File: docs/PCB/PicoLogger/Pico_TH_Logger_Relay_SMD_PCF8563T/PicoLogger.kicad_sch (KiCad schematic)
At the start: 63 parts, among them J1 Sensor, J2 LCD 16x2, J3 Additional connector, J4 K4_Output, J5 K3_Output, J6 K2_Output, J7 K1_Output, J8 SPI, K1 G5Q-1, K2 G5Q-1, K3 G5Q-1, K4 G5Q-1, Q1 MMBT3904, Q2 MMBT3904, Q3 MMBT3904, Q4 MMBT3904, SW1 SW_Push, SW2 SW_Push, U1 LTV-817S, U2 LTV-817S, U3 LTV-817S, U4 LTV-817S, U5 PCF8563T, Y1 Crystal

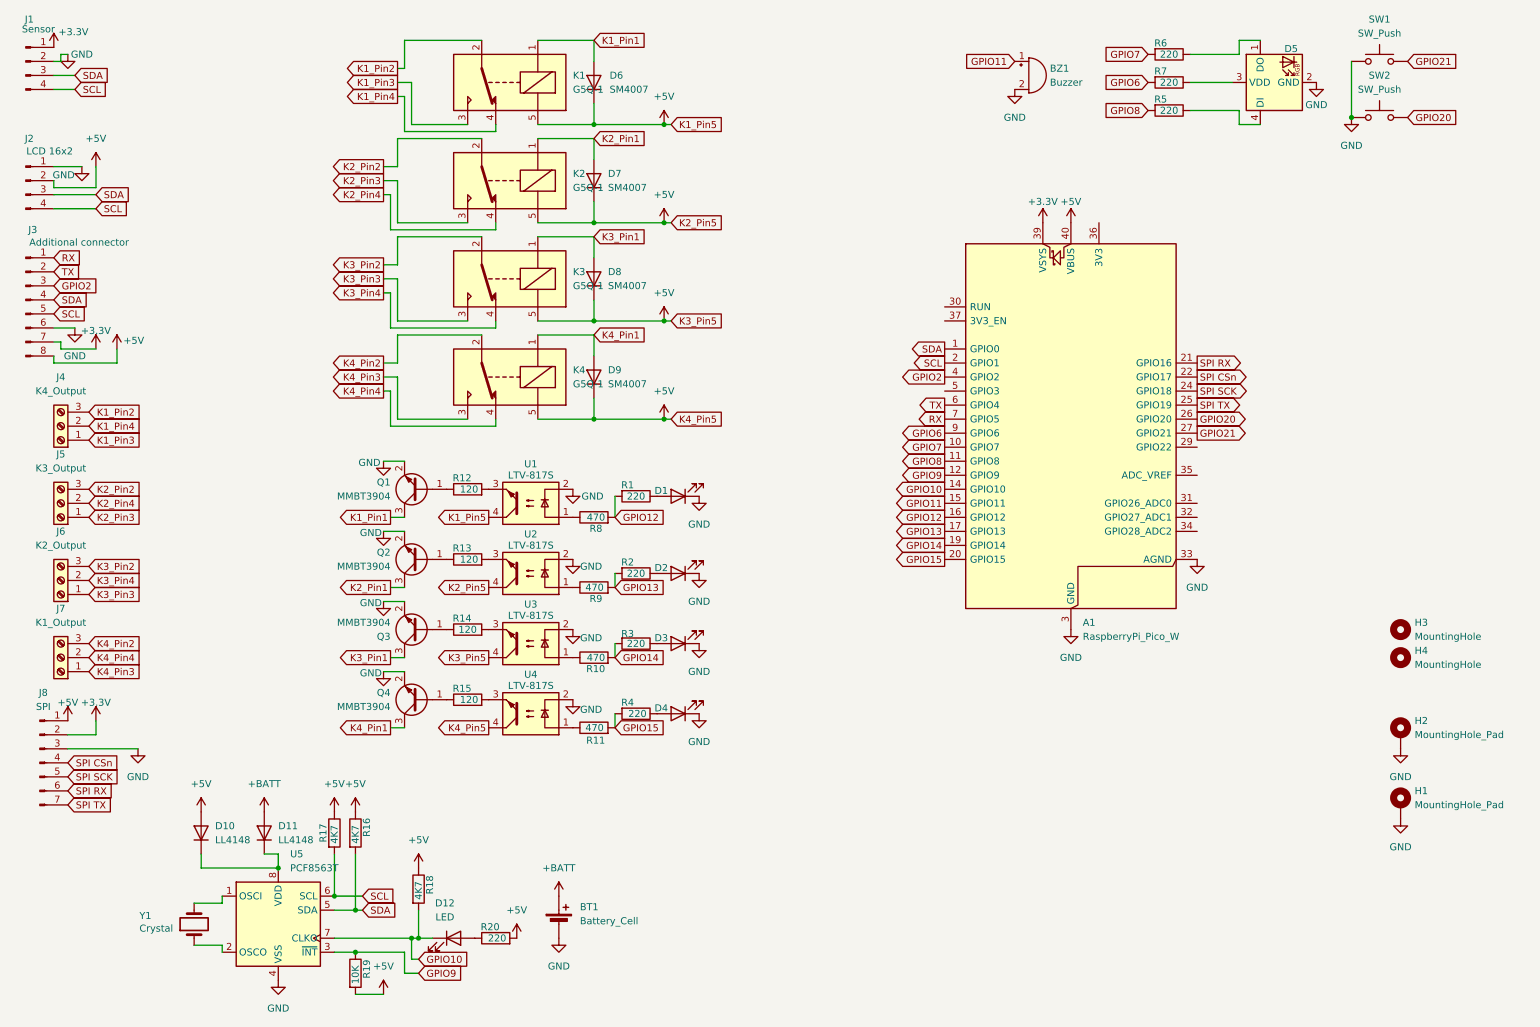
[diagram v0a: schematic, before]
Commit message: Updated docs.
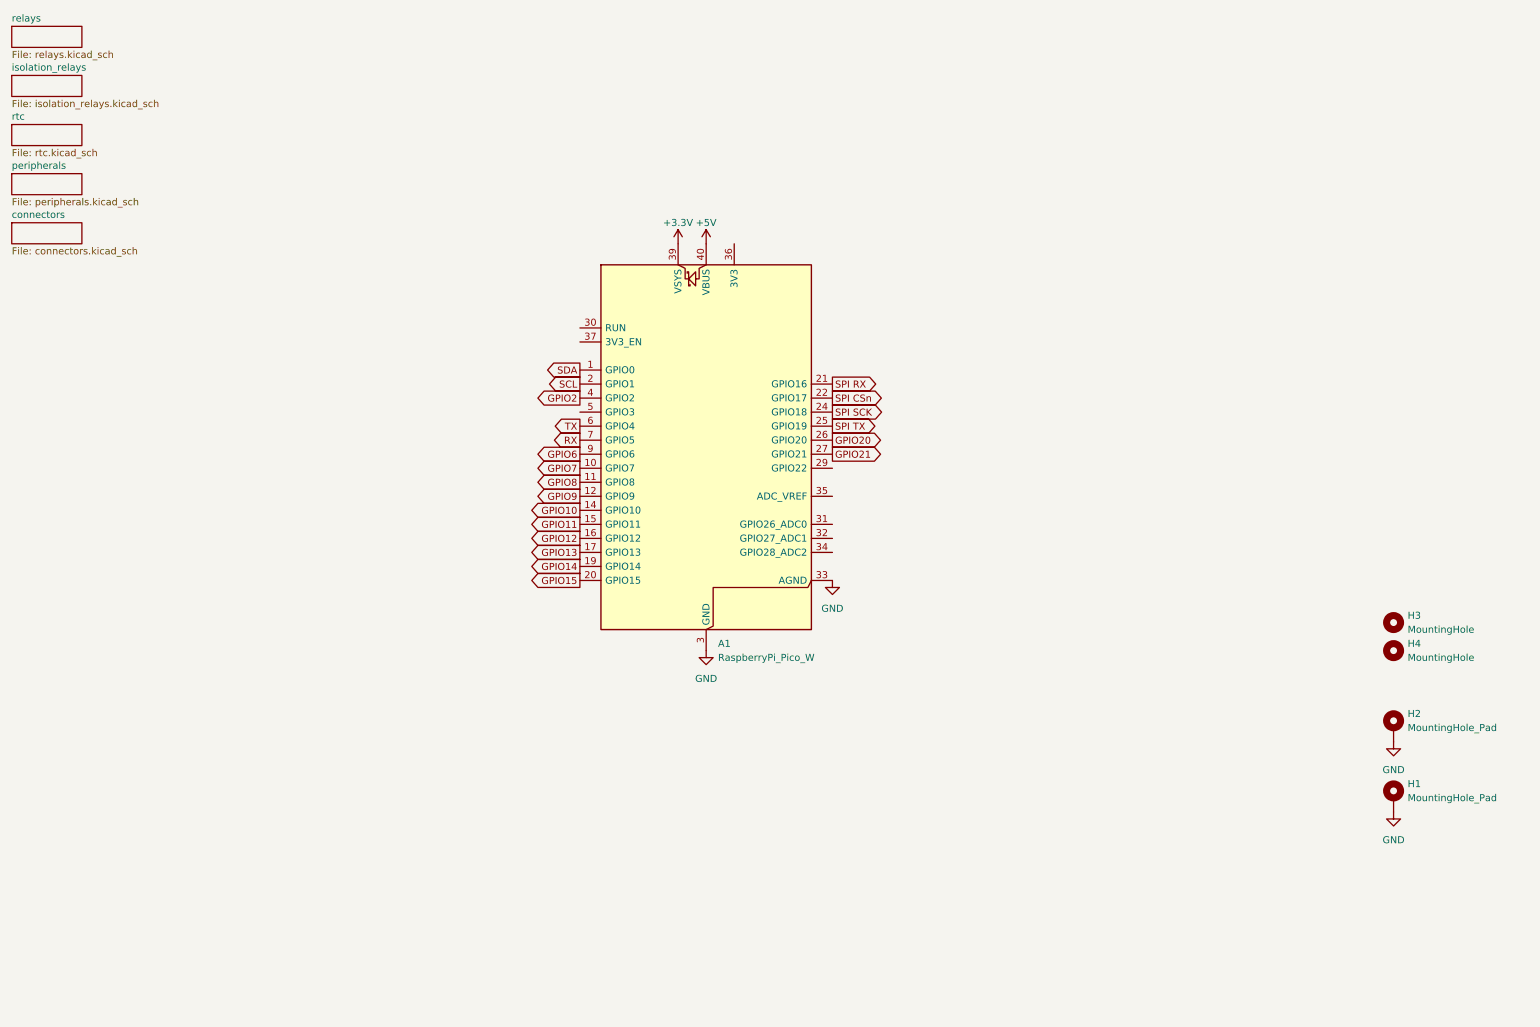
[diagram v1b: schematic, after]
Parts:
- removed BT1: Battery_Cell, Battery:BatteryHolder_Keystone_104_1x23mm, symbol Device:Battery_Cell
- removed BZ1: Buzzer, Buzzer_Beeper:Buzzer_12x9.5RM7.6, symbol Device:Buzzer
- removed D1, D12, D2, D3, D4: LED, LED_SMD:LED_0805_2012Metric, symbol Device:LED
- removed D10, D11: LL4148, Diode_SMD:D_MiniMELF, symbol Diode:LL4148
- removed D5: APA-106-F5, LED_SMD:LED_Avago_PLCC4_3.2x2.8mm_CW, symbol LED:APA-106-F5
- removed D6, D7, D8, D9: SM4007, Diode_SMD:D_SMA, symbol Diode:SM4007
- removed J1: Sensor, Connector_PinHeader_2.54mm:PinHeader_1x04_P2.54mm_Vertical, symbol Connector:Conn_01x04_Pin
- removed J2: LCD 16x2, Connector_PinHeader_2.54mm:PinHeader_1x04_P2.54mm_Vertical, symbol Connector:Conn_01x04_Pin
- removed J3: Additional connector, Connector_PinHeader_2.54mm:PinHeader_1x08_P2.54mm_Horizontal, symbol Connector:Conn_01x08_Pin
- removed J4: K4_Output, TerminalBlock_Phoenix:TerminalBlock_Phoenix_MKDS-1,5-3_1x03_P5.00mm_Horizontal, symbol Connector:Screw_Terminal_01x03
- removed J5: K3_Output, TerminalBlock_Phoenix:TerminalBlock_Phoenix_MKDS-1,5-3_1x03_P5.00mm_Horizontal, symbol Connector:Screw_Terminal_01x03
- removed J6: K2_Output, TerminalBlock_Phoenix:TerminalBlock_Phoenix_MKDS-1,5-3_1x03_P5.00mm_Horizontal, symbol Connector:Screw_Terminal_01x03
- removed J7: K1_Output, TerminalBlock_Phoenix:TerminalBlock_Phoenix_MKDS-1,5-3_1x03_P5.00mm_Horizontal, symbol Connector:Screw_Terminal_01x03
- removed J8: SPI, Connector_PinHeader_2.54mm:PinHeader_1x07_P2.54mm_Horizontal, symbol Connector:Conn_01x07_Pin
- removed K1, K2, K3, K4: G5Q-1, Relay_THT:Relay_SPDT_Omron-G5Q-1, symbol Relay:G5Q-1
- removed Q1, Q2, Q3, Q4: MMBT3904, Package_TO_SOT_SMD:SOT-23, symbol Transistor_BJT:MMBT3904
- removed R1, R2, R20, R3, R4, R5, R6, R7: 220, Resistor_SMD:R_0805_2012Metric, symbol Device:R
- removed R10, R11, R8, R9: 470, Resistor_SMD:R_0805_2012Metric, symbol Device:R
- removed R12, R13, R14, R15: 120, Resistor_SMD:R_0805_2012Metric, symbol Device:R
- removed R16, R17, R18: 4K7, Resistor_SMD:R_0805_2012Metric, symbol Device:R
- removed R19: 10K, Resistor_SMD:R_0805_2012Metric, symbol Device:R
- removed SW1, SW2: SW_Push, Button_Switch_THT:SW_PUSH_6mm, symbol Switch:SW_Push
- removed U1, U2, U3, U4: LTV-817S, Package_DIP:SMDIP-4_W9.53mm, symbol Isolator:LTV-817S
- removed U5: PCF8563T, Package_SO:SOIC-8_3.9x4.9mm_P1.27mm, symbol Timer_RTC:PCF8563T
- removed Y1: Crystal, Crystal:Crystal_SMD_3215-2Pin_3.2x1.5mm, symbol Device:Crystal
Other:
- added sheet connectors (connectors.kicad_sch)
- added sheet isolation_relays (isolation_relays.kicad_sch)
- added sheet peripherals (peripherals.kicad_sch)
- added sheet relays (relays.kicad_sch)
- added sheet rtc (rtc.kicad_sch)
- moved on the sheet: A1, H1, H2, H3, H4
